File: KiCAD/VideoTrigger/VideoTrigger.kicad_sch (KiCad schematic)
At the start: 14 parts

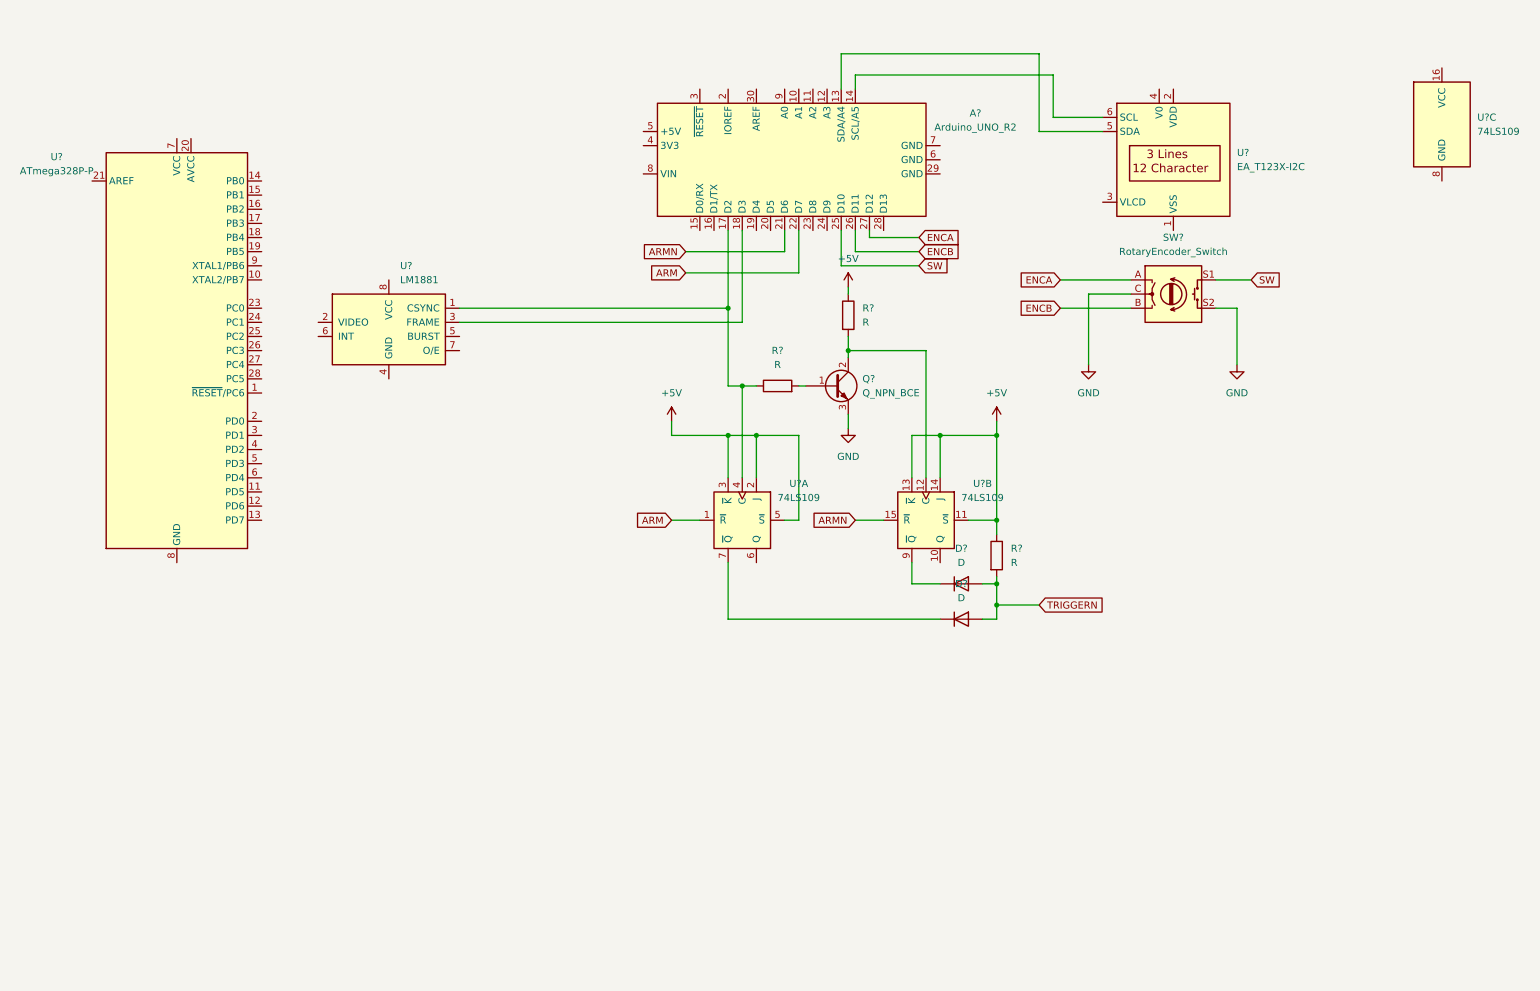
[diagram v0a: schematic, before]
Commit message: Updated README and schematic
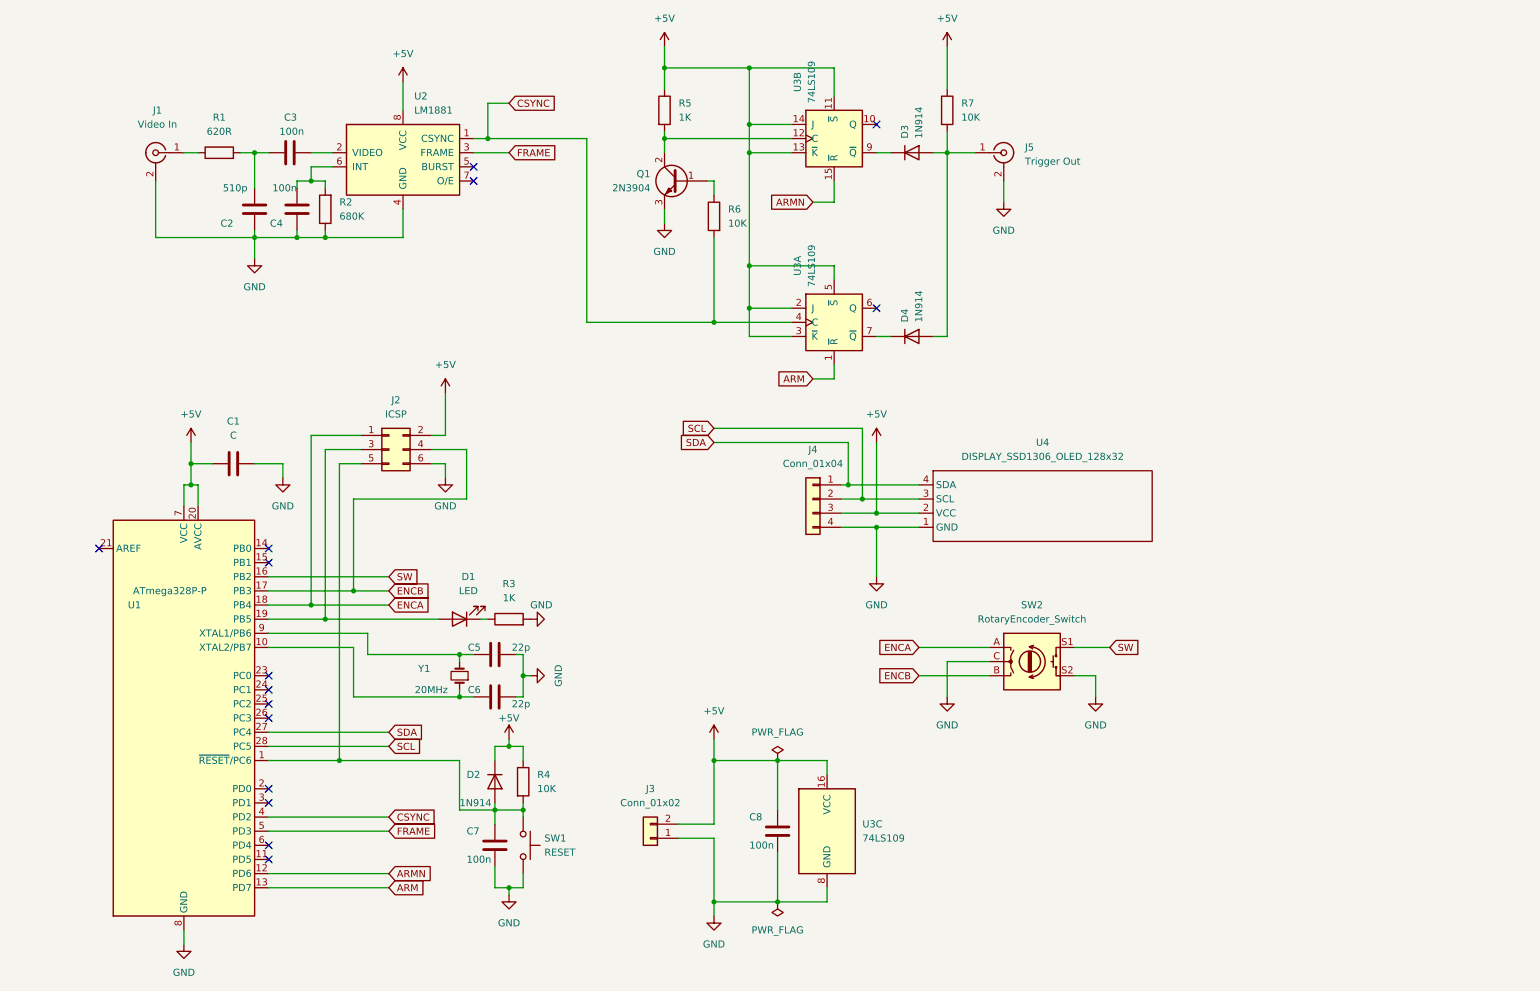
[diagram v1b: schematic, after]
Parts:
- removed A?: Arduino_UNO_R2, Module:Arduino_UNO_R2, symbol MCU_Module:Arduino_UNO_R2
- removed D? (x2): D, symbol Device:D
- removed Q?: Q_NPN_BCE, symbol Device:Q_NPN_BCE
- removed R? (x2): R, symbol Device:R
- removed U? (x2): 74LS109, symbol 74xx:74LS109
- removed U?: EA_T123X-I2C, Display:EA_T123X-I2C, symbol Display_Character:EA_T123X-I2C
- added C1: C, symbol Device:C
- added C2: 510p, symbol Device:C
- added C3, C4, C7, C8: 100n, symbol Device:C
- added C5, C6: 22p, symbol Device:C
- added D1: LED, symbol Device:LED
- added D2, D3, D4: 1N914, symbol Device:D
- added J1: Video In, symbol Connector:Conn_Coaxial
- added J2: ICSP, symbol Connector_Generic:Conn_02x03_Odd_Even
- added J3: Conn_01x02, symbol Connector_Generic:Conn_01x02
- added J4: Conn_01x04, symbol Connector_Generic:Conn_01x04
- added J5: Trigger Out, symbol Connector:Conn_Coaxial
- added Q1: 2N3904, symbol Device:Q_NPN_BCE
- added R1: 620R, symbol Device:R
- added R2: 680K, symbol Device:R
- added R3, R5: 1K, symbol Device:R
- added R4, R6: 10K, symbol Device:R
- added SW1: RESET, symbol Switch:SW_Push
- added unit 2 of U3
- added unit 1 of U3
- added U4: DISPLAY_SSD1306_OLED_128x32, symbol UKMaker:DISPLAY_SSD1306_OLED_128x32
- added Y1: 20MHz, symbol Device:Crystal_Small
- R7: renamed from R?; value R -> 10K
- gave numbers to parts that had none: 4
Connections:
- net +5V: now also U1.20 (AVCC), U1.7 (VCC), U2.8 (VCC), U3.16 (VCC), C1.1, C8.1, D2.1 (K), J2.2 (Pin_2), J3.2 (Pin_2), J4.3 (Pin_3), R4.1, R5.1, U3.11 (~{S}), U3.13 (~{K}), U3.14 (J), U3.2 (J), U3.3 (~{K}), U3.5 (~{S}), U4.2 (VCC)
- net ARM: now also U1.13 (PD7), U3.1 (~{R})
- net ARMN: now also U1.12 (PD6), U3.15 (~{R})
- net ENCA: now also U1.18 (PB4), J2.1 (Pin_1)
- net ENCB: now also U1.17 (PB3), J2.4 (Pin_4)
- net GND: now also U1.22 (GND), U1.8 (GND), U2.4 (GND), U3.8 (GND), C1.2, C2.2, C4.2, C5.1, C6.1, C7.2, C8.2, J1.2 (Ext), J2.6 (Pin_6), J3.1 (Pin_1), J4.4 (Pin_4), J5.2 (Ext), Q1.3 (E), R2.1, R3.2, SW1.2, U4.1 (GND)
- net SW: now also U1.16 (PB2)
- net CSYNC: now reaches U2.1 (CSYNC)
- net CSYNC: now also U1.4 (PD2), R6.2, U3.4 (C)
- net FRAME: now reaches U2.3 (FRAME)
- net FRAME: now also U1.5 (PD3)
- net at U2.2 (VIDEO): now also C3.1
- net at U2.6 (INT): now also C4.1, R2.2
- net at U1.1 (~{RESET}/PC6): now also C7.1, D2.2 (A), J2.5 (Pin_5), R4.2, SW1.1
- net at U1.10 (XTAL2/PB7): now also C6.2, Y1.1
- net at U1.19 (PB5): now also D1.2 (A), J2.3 (Pin_3)
- net SDA: now reaches U1.27 (PC4)
- net SDA: now also J4.1 (Pin_1), U4.4 (SDA)
- net SCL: now reaches U1.28 (PC5)
- net SCL: now also J4.2 (Pin_2), U4.3 (SCL)
- net at U1.9 (XTAL1/PB6): now also C5.2, Y1.2
- net TRIGGERN: no longer names the net of R7.2
- net TRIGGERN: now also D3.2 (A), D4.2 (A), J5.1 (In)
- new net: Q1.2 (C), R5.2, U3.12 (C)
- new net: D3.1 (K), U3.9 (~{Q})
- new net: Q1.1 (B), R6.1
- new net: C2.1, C3.2, R1.2
- new net: D4.1 (K), U3.7 (~{Q})
- new net: D1.1 (K), R3.1
- new net: J1.1 (In), R1.1
- no-connect marks 0 -> 15
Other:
- company: (none) -> Duncan McIntyre (UKMaker)
- title: (none) -> Video Trigger
- moved on the sheet: R7, SW2, U1, U2, U3C
